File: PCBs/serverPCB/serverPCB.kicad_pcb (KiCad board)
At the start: 2 copper layers, 45.7 x 61 mm, 5 parts

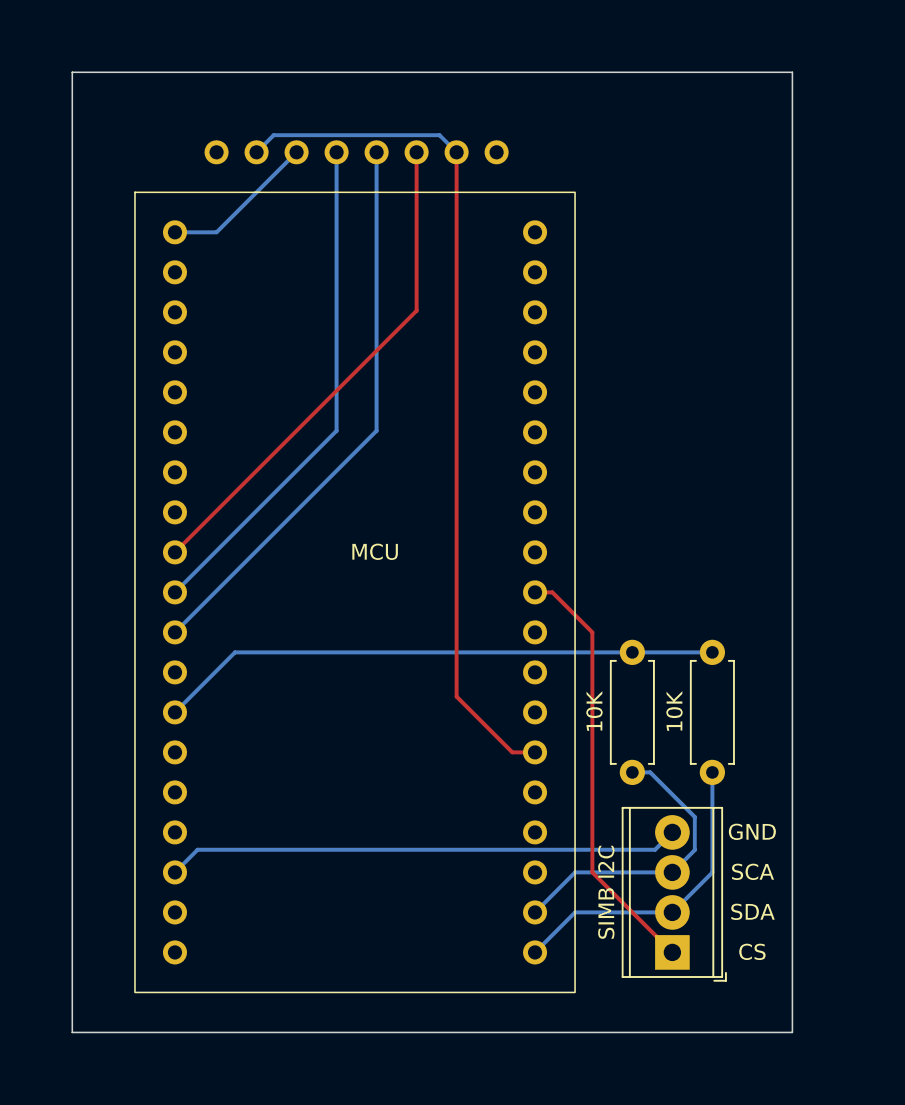
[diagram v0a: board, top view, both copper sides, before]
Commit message: pcb edits
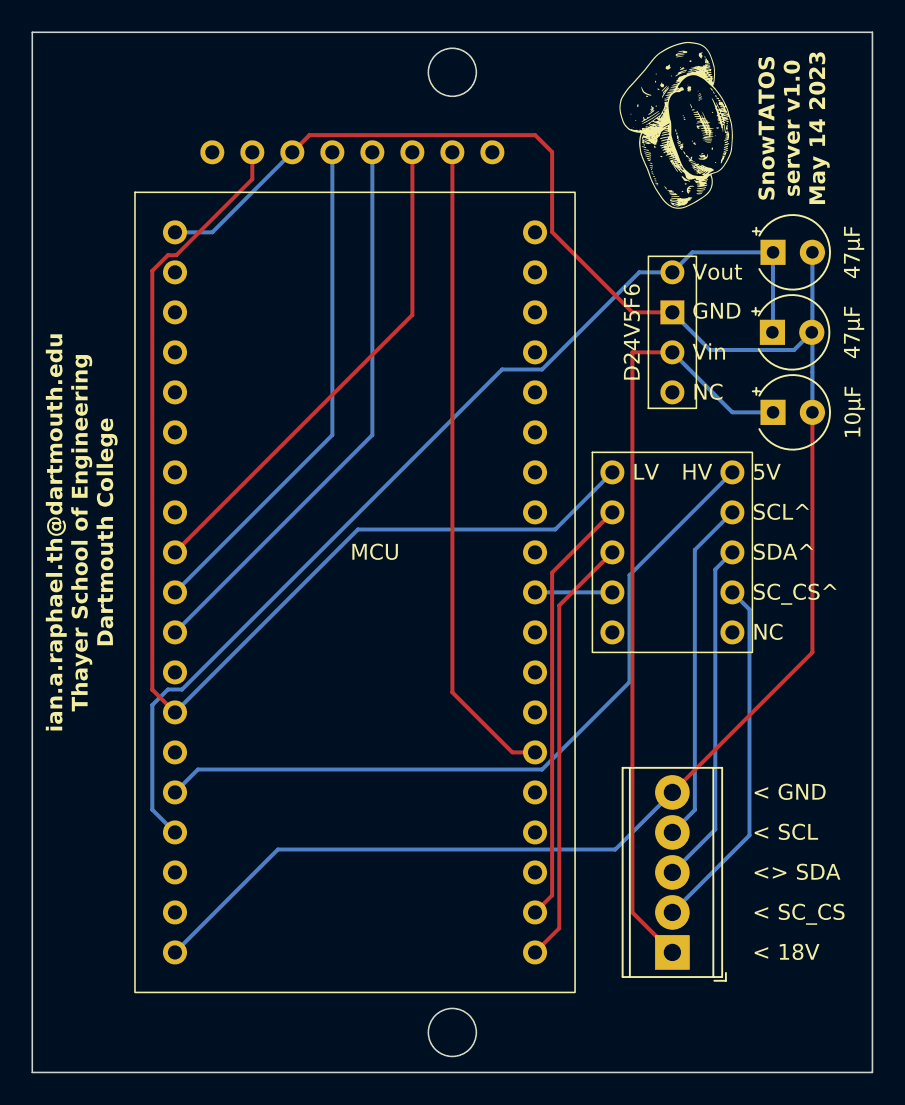
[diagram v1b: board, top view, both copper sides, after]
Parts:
- removed 10K (x2): 10K, Resistor_THT:R_Axial_DIN0207_L6.3mm_D2.5mm_P7.62mm_Horizontal
- added C1: 10µF, Capacitor_THT:CP_Radial_Tantal_D4.5mm_P2.50mm, F.Cu at (161.3, 82.5)
- added C2: 47µF, Capacitor_THT:CP_Radial_Tantal_D4.5mm_P2.50mm, F.Cu at (161.3, 77.5)
- added C3: 47µF, Capacitor_THT:CP_Radial_Tantal_D4.5mm_P2.50mm, F.Cu at (161.3, 72.4)
- added G***: LOGO, LOGO, F.Cu at (154.9, 64.3)
- added U1: TPSM84203, Converter_DCDC:Pololu_D24V5F9, F.Cu at (154.9, 77.7)
- added U2: ~, Converter_DCDC:Pololu_logicLevelShifter, F.Cu at (154.9, 91.4)
- J1: renamed from SIMB I2C; footprint TerminalBlock_Phoenix:TerminalBlock_Phoenix_MPT-0,5-4-2.54_1x04_P2.54mm_Horizontal -> TerminalBlock_Phoenix:TerminalBlock_Phoenix_MPT-0,5-5-2.54_1x05_P2.54mm_Horizontal
- moved µSD 1.13 mm to (134.6, 79.8)
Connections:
- J1 pad 4: /GND -> Net-(J1-Pin_4)
- MCU pad 20: Net-(J1-Pin_2) -> Net-(MCU1-SDA)
- MCU pad 21: Net-(J1-Pin_3) -> Net-(MCU1-SCL)
- MCU pad 5V: unconnected-(MCU1-Pad5V) -> /5V
- MCU pad 6: Net-(J1-Pin_1) -> Net-(MCU1-D6)
- MCU pad VIN: unconnected-(MCU1-PadVIN) -> Net-(U1-Vout)
- µSD pad 7: /sd_cs -> /3V3
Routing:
- net /GND: track 42.5 -> 125.8 mm
- net Net-(U1-Vout): track 0.00 -> 65.0 mm
- net /5V: track 0.00 -> 47.8 mm
- net /3V3: track 35.7 -> 73.2 mm
- net Net-(MCU1-SDA): track 0.00 -> 27.4 mm
- net Net-(MCU1-SCL): track 0.00 -> 27.4 mm
- net Net-(J1-Pin_1): track 27.1 -> 49.7 mm
- net Net-(J1-Pin_4): track 0.00 -> 21.9 mm
- net /sd_cs: track 54.6 -> 41.1 mm
- net Net-(MCU1-D6): track 0.00 -> 4.91 mm
- net Net-(J1-Pin_2): track 19.7 -> 22.8 mm
- net Net-(J1-Pin_3): track 19.0 -> 21.9 mm
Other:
- board size 45.7 x 61 mm -> 53.3 x 66 mm
- board text added: "5V"
- board text added: "< 18V"
- board text added: "< GND"
- board text added: "< SCL"
- board text added: "< SC_CS"
- board text added: "<> SDA"
- board text added: "D24V5F6"
- board text added: "HV"
- board text added: "LV"
- board text added: "NC"
- board text added: "SCL^"
- board text added: "SC_CS^"
- board text added: "SDA^"
- board text added: "SnowTATOS server v1.0 May 14 2023"
- board text added: "Vin"
- board text added: "Vout"
- board text added: "ian.a.raphael.th@dartmouth.edu Thayer School of Engineering Dartmouth College"
- board text removed: "CS"
- board text removed: "SCA"
- board text removed: "SDA"
